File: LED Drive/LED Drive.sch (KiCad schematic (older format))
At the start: 0 parts

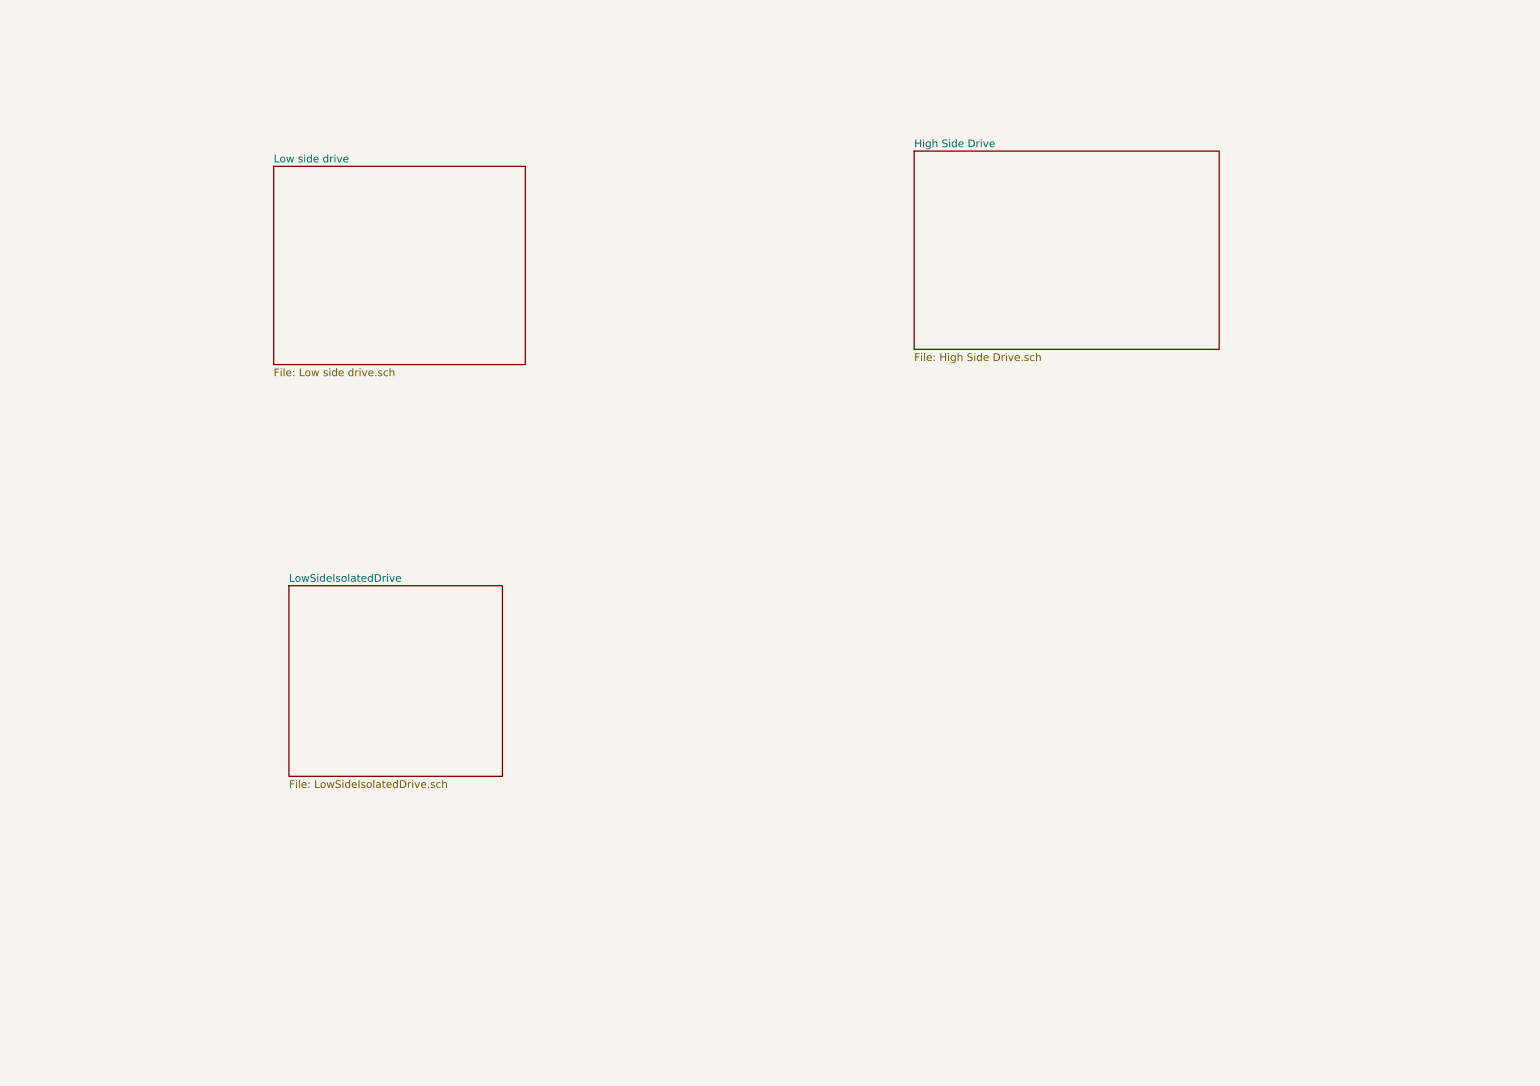
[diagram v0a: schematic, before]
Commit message: 9-8
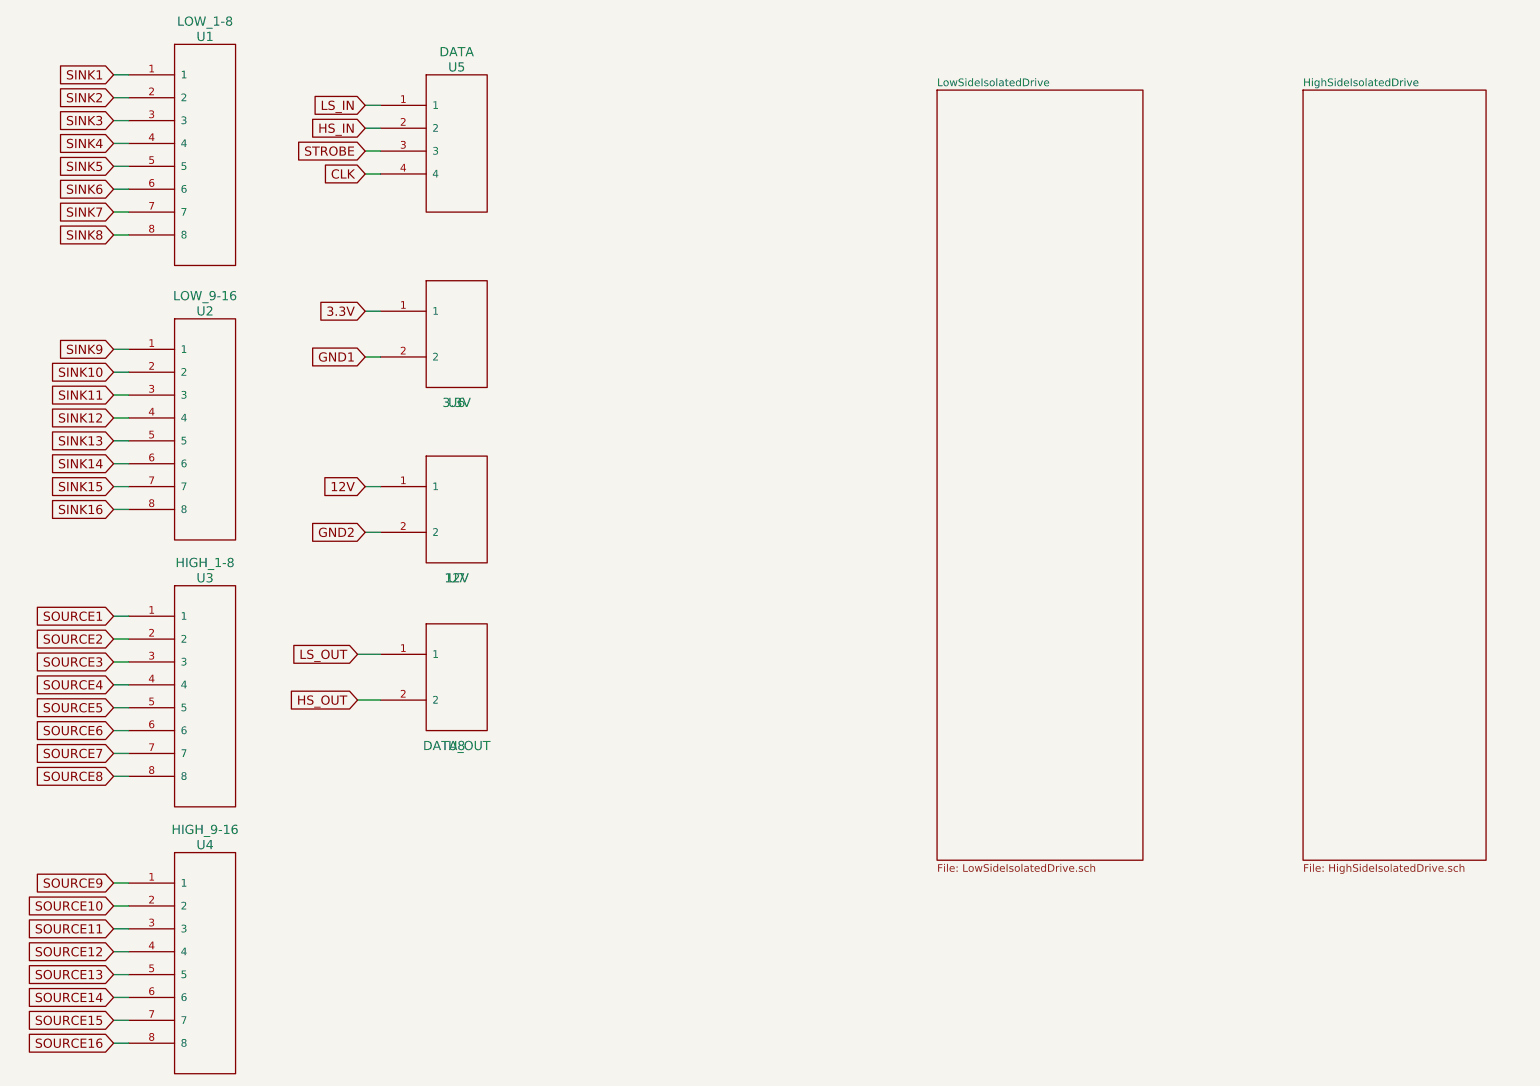
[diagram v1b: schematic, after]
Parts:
- added U1: LOW_1-8, ~, symbol WIRE8
- added U2: LOW_9-16, ~, symbol WIRE8
- added U3: HIGH_1-8, ~, symbol WIRE8
- added U4: HIGH_9-16, ~, symbol WIRE8
- added U5: DATA, ~, symbol WIRE4
- added U6: 3.3V, ~, symbol WIRE2
- added U7: 12V, ~, symbol WIRE2
- added U8: DATA_OUT, ~, symbol WIRE2
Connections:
- new net 12V: U7.1
- new net 3.3V: U6.1
- new net CLK: U5.4
- new net GND1: U6.2
- new net GND2: U7.2
- new net HS_IN: U5.2
- new net HS_OUT: U8.2
- new net LS_IN: U5.1
- new net LS_OUT: U8.1
- new net SINK1: U1.1
- new net SINK10: U2.2
- new net SINK11: U2.3
- new net SINK12: U2.4
- new net SINK13: U2.5
- new net SINK14: U2.6
- new net SINK15: U2.7
- new net SINK16: U2.8
- new net SINK2: U1.2
- new net SINK3: U1.3
- new net SINK4: U1.4
- new net SINK5: U1.5
- new net SINK6: U1.6
- new net SINK7: U1.7
- new net SINK8: U1.8
- new net SINK9: U2.1
- new net SOURCE1: U3.1
- new net SOURCE10: U4.2
- new net SOURCE11: U4.3
- new net SOURCE12: U4.4
- new net SOURCE13: U4.5
- new net SOURCE14: U4.6
- new net SOURCE15: U4.7
- new net SOURCE16: U4.8
- new net SOURCE2: U3.2
- new net SOURCE3: U3.3
- new net SOURCE4: U3.4
- new net SOURCE5: U3.5
- new net SOURCE6: U3.6
- new net SOURCE7: U3.7
- new net SOURCE8: U3.8
- new net SOURCE9: U4.1
- new net STROBE: U5.3
